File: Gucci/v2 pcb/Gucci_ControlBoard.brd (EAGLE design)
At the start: 66 x 56 mm, 57 parts, among them U1 PCA9306_LSSOP, U2 TEENSY_3.6_DIL, U5 LM393-8-SOIC, U6 AP2114H-1.8TRG1, U7 AP2114H-3.3TRG1

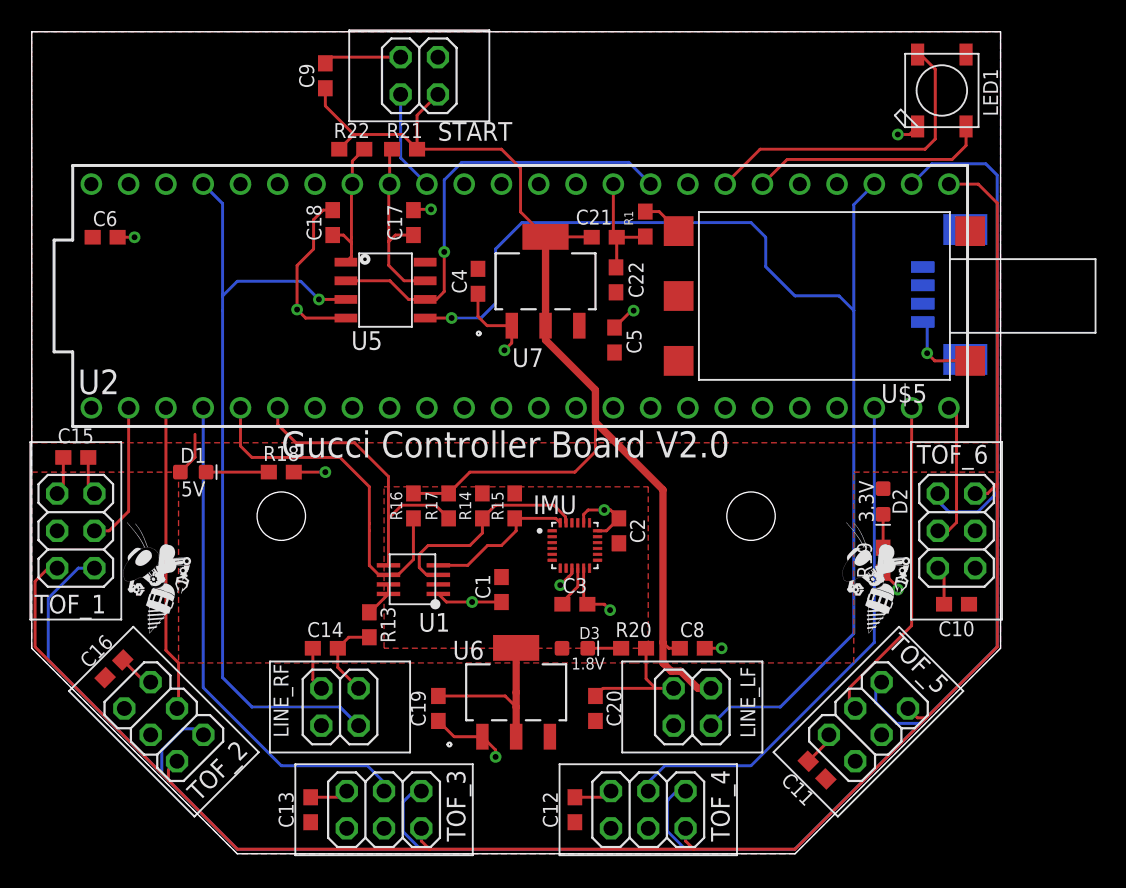
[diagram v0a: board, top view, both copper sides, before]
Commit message: Moved LEDs and NeoPixel to bottom
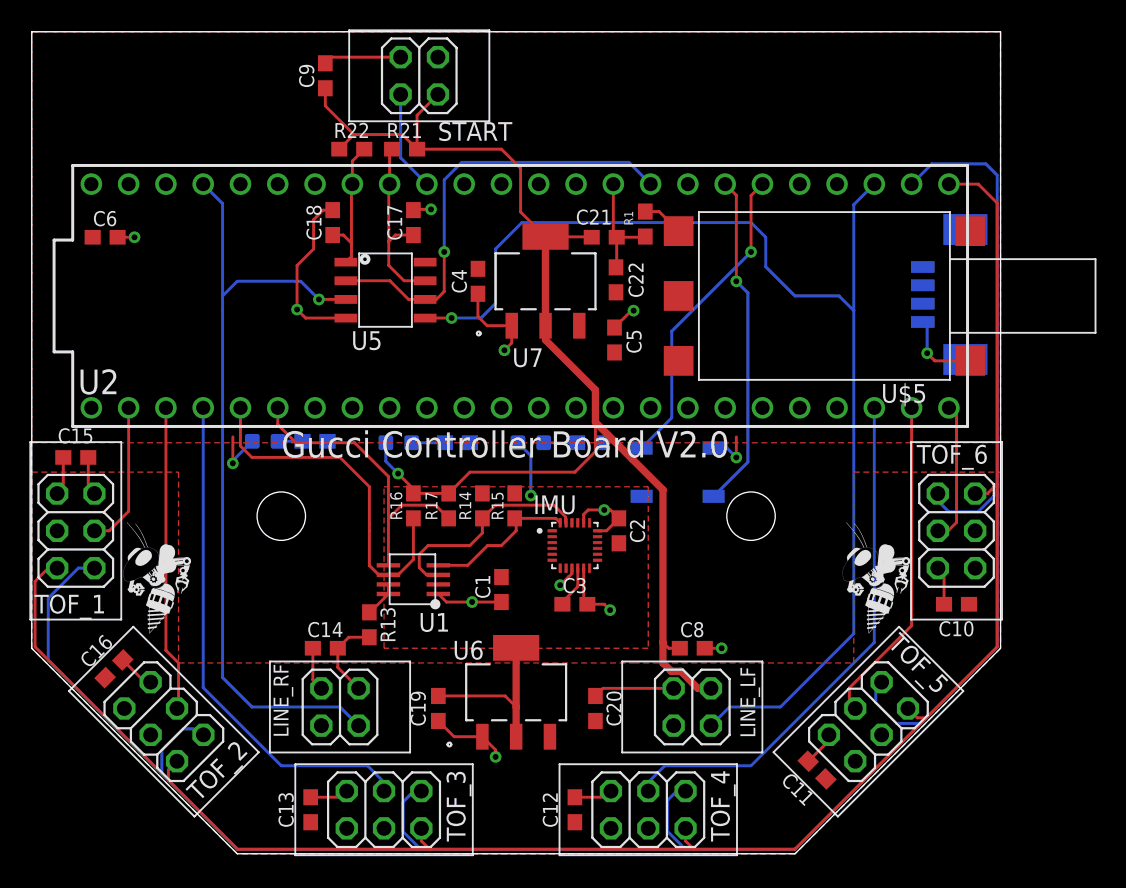
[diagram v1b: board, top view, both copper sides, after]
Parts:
- moved D2 33.2 mm to (11.0, 28.0), flipped to the bottom, turned to 180 degrees
- moved LED1 31.6 mm to (30.0, 26.0), flipped to the bottom, turned to 180 degrees
- moved R19 30.1 mm to (15.0, 28.0), flipped to the bottom, turned to 180 degrees
- moved D3 14.3 mm to (20.0, 28.0), flipped to the bottom, turned to 180 degrees
- moved R20 14.3 mm to (24.0, 28.0), flipped to the bottom, turned to 180 degrees
- moved D1 5.33 mm to (1.90, 28.1), flipped to the bottom, turned to 180 degrees
- moved R18 3.11 mm to (5.30, 28.1), flipped to the bottom, turned to 180 degrees
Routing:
- net GND: track 89.0 -> 80.7 mm, vias 14 -> 11
- net NEO_DI: track 16.3 -> 21.4 mm, vias 0 -> 1
- net 3.3V: track 92.2 -> 96.4 mm, vias 0 -> 1
- net 5V: track 2.99 -> 7.07 mm, vias 0 -> 2
- net 1.8V: track 11.7 -> 15.6 mm, vias 0 -> 1
- net N$1: track 4.27 -> 1.67 mm
- net NEO_DO: track 22.0 -> 22.9 mm, vias 0 -> 1
